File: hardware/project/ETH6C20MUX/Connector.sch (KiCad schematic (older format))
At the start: 9 parts, among them J501 Conn_01x06, J502 Conn_02x08_Odd_Even, J503 C64AC

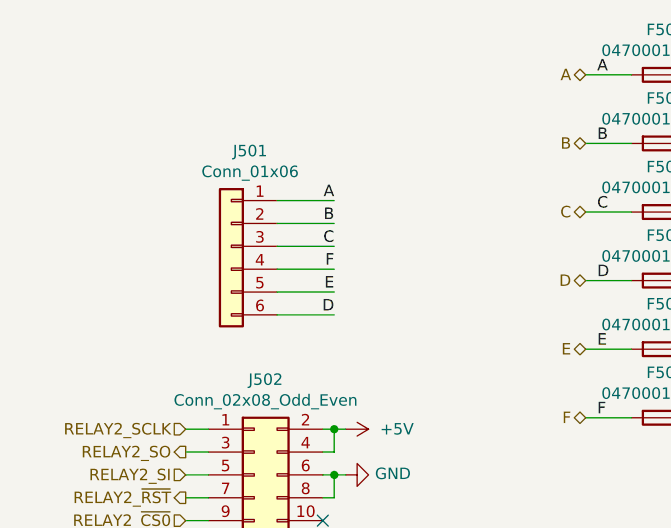
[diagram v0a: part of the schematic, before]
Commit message: PCB design
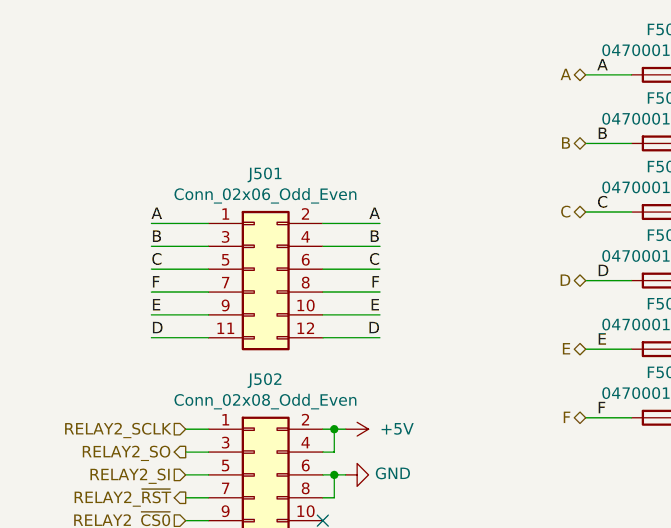
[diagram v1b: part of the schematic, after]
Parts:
- removed J501: Conn_01x06, Connector_PinSocket_2.54mm:PinSocket_1x06_P2.54mm_Vertical, symbol Connector_Generic:Conn_01x06
- added J501: Conn_02x06_Odd_Even, Connector_PinSocket_2.54mm:PinSocket_2x06_P2.54mm_Vertical, symbol Connector_Generic:Conn_02x06_Odd_Even
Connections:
- net A: now also J501.1 (Pin_1), J501.2 (Pin_2)
- net B: now also J501.3 (Pin_3), J501.4 (Pin_4)
- net C: now also J501.5 (Pin_5), J501.6 (Pin_6)
- net D: now also J501.11 (Pin_11), J501.12 (Pin_12)
- net E: now also J501.10 (Pin_10), J501.9 (Pin_9)
- net F: now also J501.7 (Pin_7), J501.8 (Pin_8)
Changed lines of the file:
@@
 	0    1    1    0
 $EndComp
-Text Label 3500 1300 2    50   ~ 0
+Text Label 3700 1400 2    50   ~ 0
 A
-Text Label 3500 1400 2    50   ~ 0
+Text Label 3700 1500 2    50   ~ 0
 B
-Text Label 3500 1500 2    50   ~ 0
+Text Label 3700 1600 2    50   ~ 0
 C
-Text Label 3500 1800 2    50   ~ 0
+Text Label 3700 1900 2    50   ~ 0
 D
-Text Label 3500 1700 2    50   ~ 0
+Text Label 3700 1800 2    50   ~ 0
 E
-Text Label 3500 1600 2    50   ~ 0
+Text Label 3700 1700 2    50   ~ 0
 F
-$Comp
-L Connector_Generic:Conn_01x06 J?
-U 1 1 5D777B7C
-P 3050 1500
-AR Path="/5D7599BA/5D777B7C" Ref="J?"  Part="1"
-AR Path="/5DB25E5A/5D777B7C" Ref="J501"  Part="1"
-F 0 "J501" H 2968 1917 50  0000 C CNN
-F 1 "Conn_01x06" H 2968 1826 50  0000 C CNN
-F 2 "Connector_PinSocket_2.54mm:PinSocket_1x06_P2.54mm_Vertical" H 3050 1500 50  0001 C CNN
-F 3 "~" H 3050 1500 50  0001 C CNN
-	1    3050 1500
-	-1   0    0    -1
-$EndComp
-Wire Wire Line
-	3250 1300 3500 1300
-Wire Wire Line
-	3250 1400 3500 1400
-Wire Wire Line
-	3250 1500 3500 1500
-Wire Wire Line
-	3250 1800 3500 1800
-Wire Wire Line
-	3250 1700 3500 1700
-Wire Wire Line
-	3250 1600 3500 1600
+Wire Wire Line
+	3450 1400 3700 1400
+Wire Wire Line
+	3450 1500 3700 1500
+Wire Wire Line
+	3450 1600 3700 1600
+Wire Wire Line
+	3450 1900 3700 1900
+Wire Wire Line
+	3450 1800 3700 1800
+Wire Wire Line
+	3450 1700 3700 1700
 NoConn ~ 5650 2200
 NoConn ~ 5650 2300
@@
 	3550 3000 3450 3000
 NoConn ~ 3450 2700
+$Comp
+L Connector_Generic:Conn_02x06_Odd_Even J501
+U 1 1 6024031A
+P 3150 1600
+F 0 "J501" H 3200 2017 50  0000 C CNN
+F 1 "Conn_02x06_Odd_Even" H 3200 1926 50  0000 C CNN
+F 2 "Connector_PinSocket_2.54mm:PinSocket_2x06_P2.54mm_Vertical" H 3150 1600 50  0001 C CNN
+F 3 "~" H 3150 1600 50  0001 C CNN
+	1    3150 1600
+	1    0    0    -1
+$EndComp
+Text Label 2700 1400 0    50   ~ 0
+A
+Text Label 2700 1500 0    50   ~ 0
+B
+Text Label 2700 1600 0    50   ~ 0
+C
+Text Label 2700 1900 0    50   ~ 0
+D
+Text Label 2700 1800 0    50   ~ 0
+E
+Text Label 2700 1700 0    50   ~ 0
+F
+Wire Wire Line
+	2950 1400 2700 1400
+Wire Wire Line
+	2950 1500 2700 1500
+Wire Wire Line
+	2950 1600 2700 1600
+Wire Wire Line
+	2950 1900 2700 1900
+Wire Wire Line
+	2950 1800 2700 1800
+Wire Wire Line
+	2950 1700 2700 1700
 $EndSCHEMATC
